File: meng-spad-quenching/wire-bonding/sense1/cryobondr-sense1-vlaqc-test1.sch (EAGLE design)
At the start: 28 parts, among them IC2 SENSE1, U2 SN74LVC1G34DCKT, X1 CONN-D3, X10 AQCR3_VDD2V5, X2 CONN-D5, X3 CONN-D4, X4 AQCR3_AV_DET, X5 AQCR3_IBIAS, X6 CONN-D6, X7 CONN-D7, X8 CONN-D8, X9 AQCR3_SPAD_CATHODE

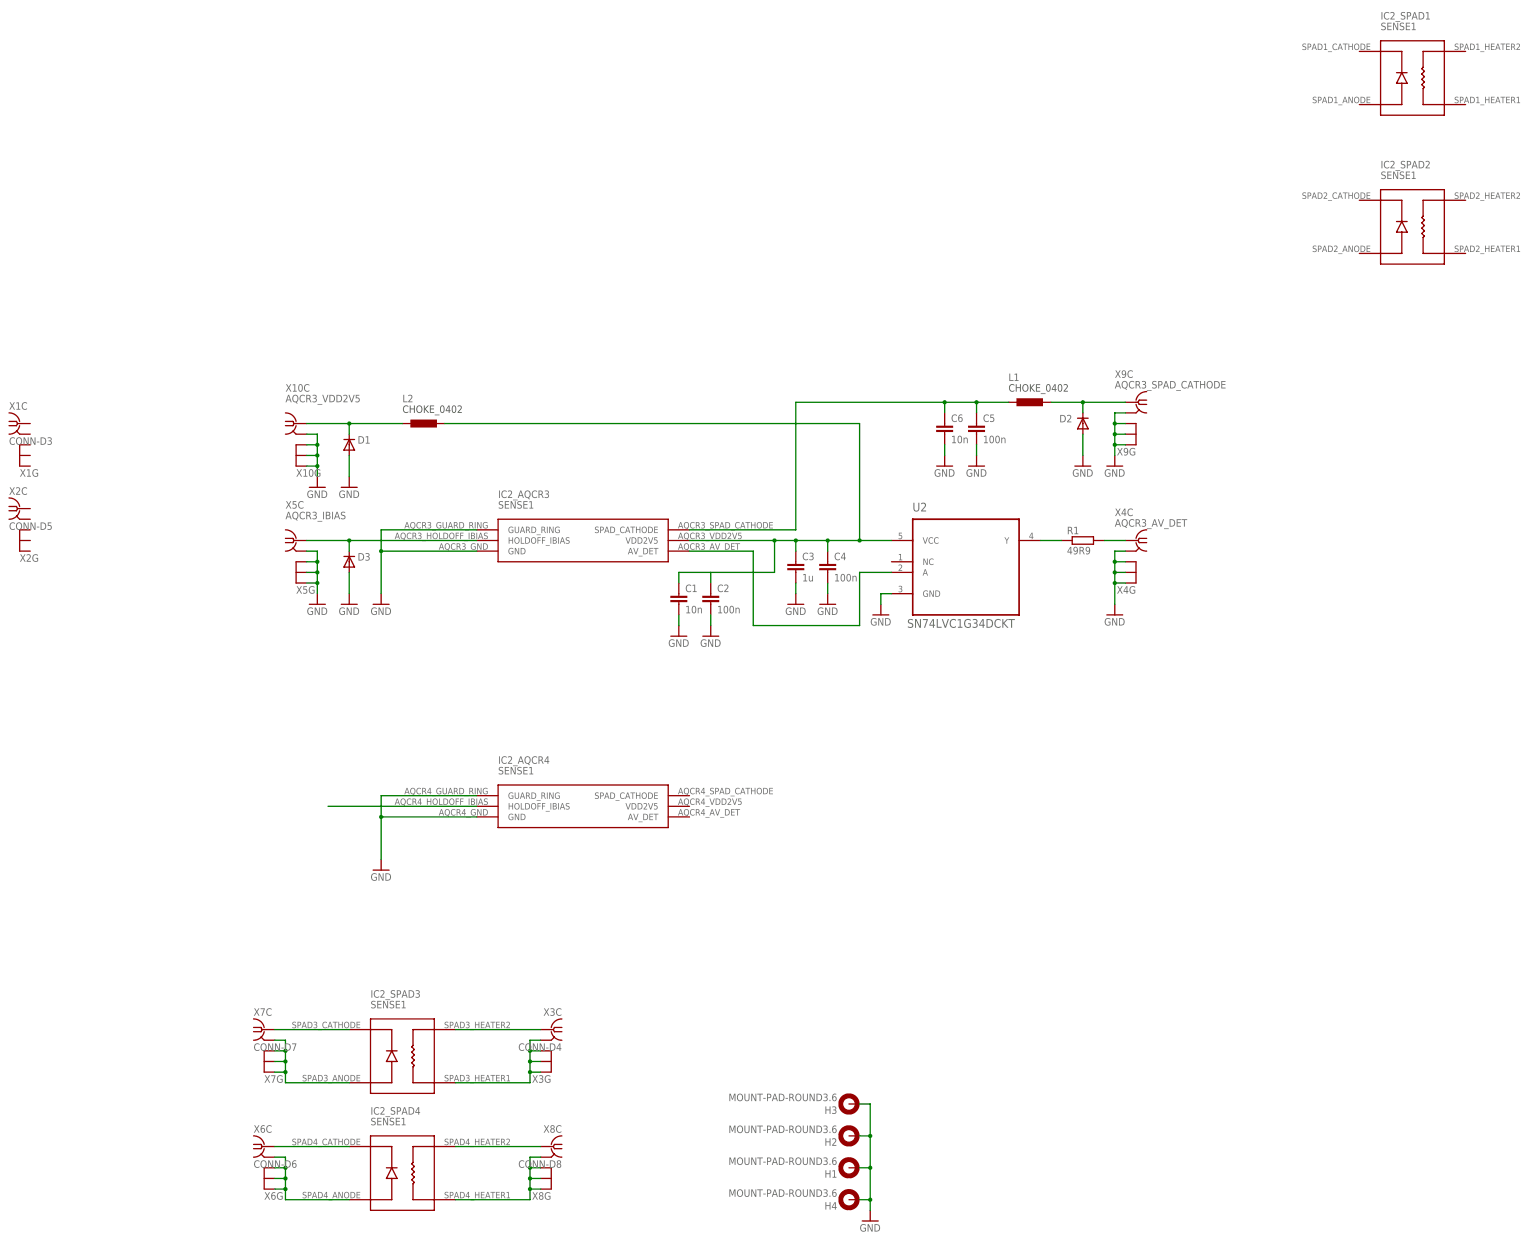
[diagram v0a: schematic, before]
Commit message: Added all MakeMIT active probe files (unsorted)
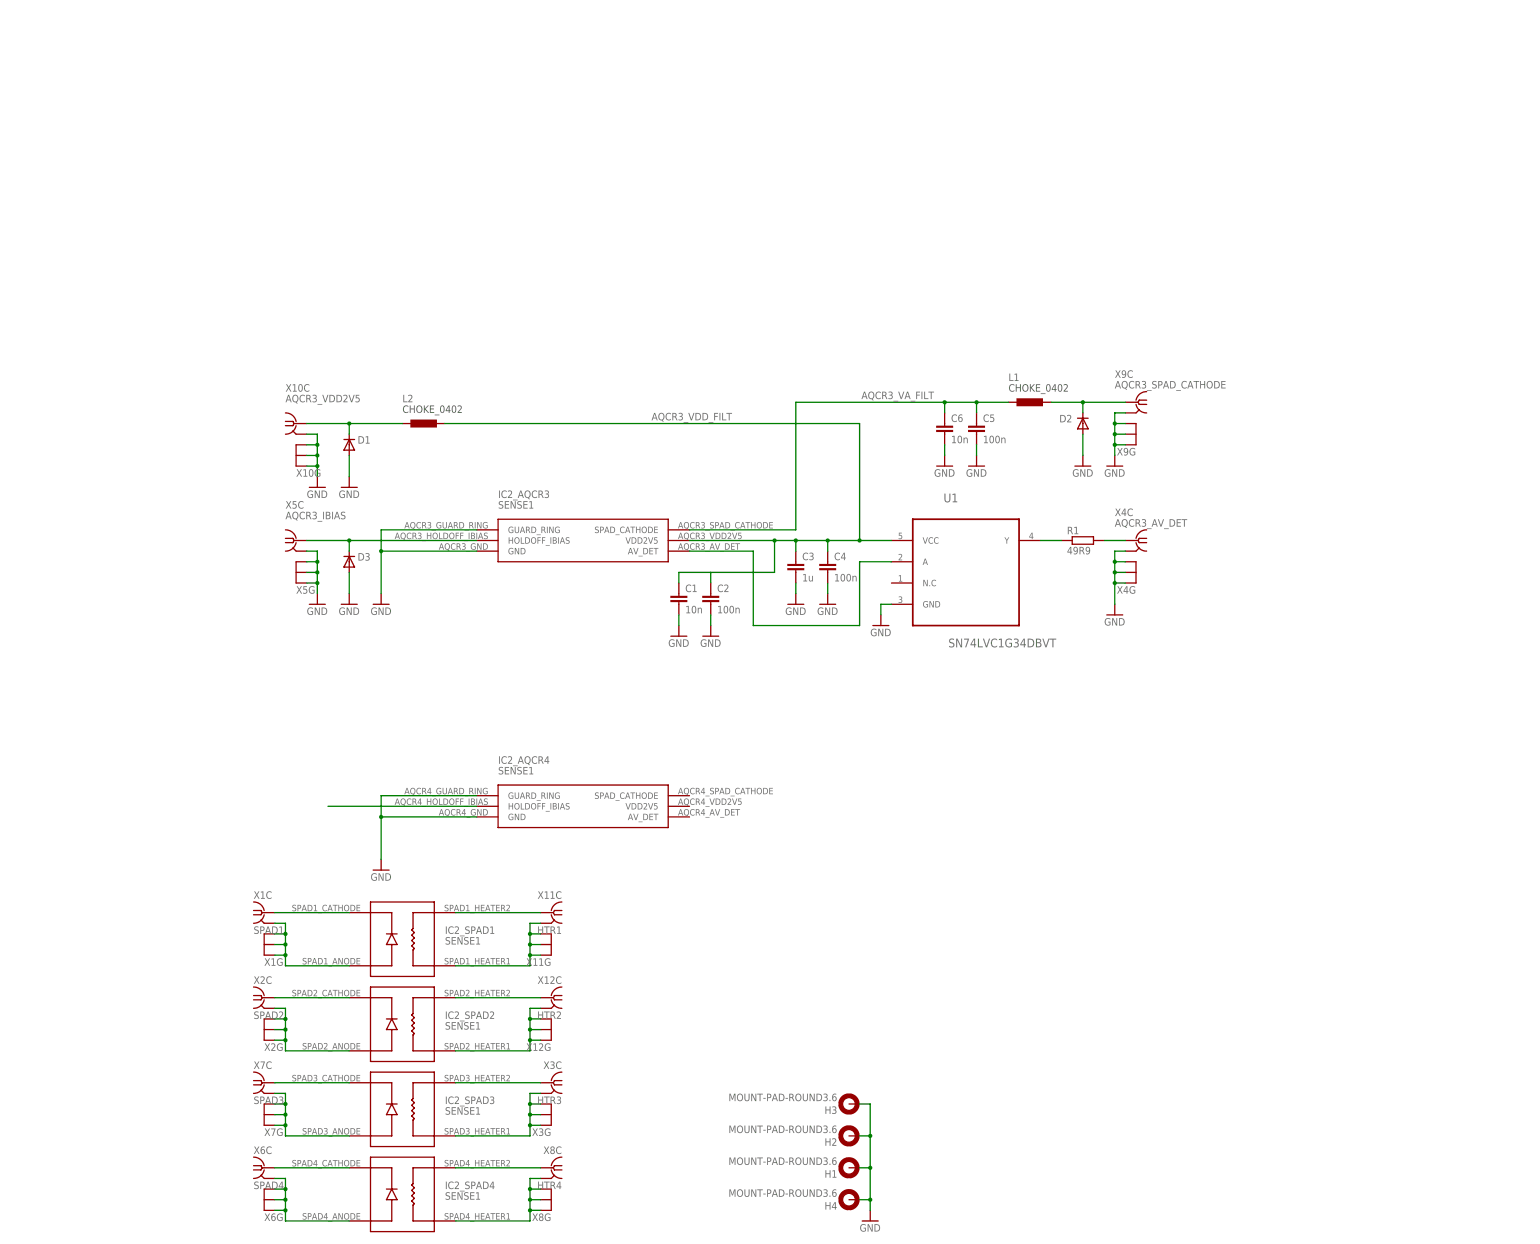
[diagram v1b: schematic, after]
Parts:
- removed U2: SN74LVC1G34DCKT, Texas Instruments_By_element14_Batch_1:SN74LVC1G34DCKT
- added U1: SN74LVC1G34DBVT, Texas Instruments_By_element14_Batch_1:SN74LVC1G34DBVT
- added X11: HTR1, meng:MMCXBIGPAD
- added X12: HTR2, meng:MMCXBIGPAD
- C1, C2, C3, C4, C5, C6: device rcl:C-EUC0402 -> rcl:C-EUC0603
- D1, D2, D3: device diode:DIODE-SOD123 -> diode:DIODE-SOD323-W
- X1: value CONN-D3 -> SPAD1
- X2: value CONN-D5 -> SPAD2
- X3: value CONN-D4 -> HTR3
- X6: value CONN-D6 -> SPAD4
- X7: value CONN-D7 -> SPAD3
- X8: value CONN-D8 -> HTR4
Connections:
- net N$8 renamed AQCR3_VA_FILT
- removed net N$9: C1.1, C2.1, C3.1, C4.1, IC2_AQCR3.VDD2V5, L2.P$2, U2.VCC
- new net AQCR3_VDD_FILT: C1.1, C2.1, C3.1, C4.1, IC2_AQCR3.VDD2V5, L2.P$2, U1.VCC
- new net N$18: IC2_SPAD2.SPAD_CATHODE, X2C.1
- new net N$19: IC2_SPAD2.SPAD_ANODE, X2C.GND, X2G.GND@1, X2G.GND@2, X2G.GND@3
- new net N$20: IC2_SPAD1.SPAD_ANODE, X1C.GND, X1G.GND@1, X1G.GND@2, X1G.GND@3
- new net N$21: IC2_SPAD1.SPAD_CATHODE, X1C.1
- new net N$22: IC2_SPAD1.SPAD_HEATER2, X11C.1
- new net N$23: IC2_SPAD2.SPAD_HEATER2, X12C.1
- new net N$24: IC2_SPAD1.SPAD_HEATER1, X11C.GND, X11G.GND@1, X11G.GND@2, X11G.GND@3
- new net N$25: IC2_SPAD2.SPAD_HEATER1, X12C.GND, X12G.GND@1, X12G.GND@2, X12G.GND@3
- net GND: now also U1.GND; no longer U2.GND
- net N$2: now also U1.Y; no longer U2.Y
- net N$7: now also U1.A; no longer U2.A
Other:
- note added: "Low-Temperature Component Guidelines: - Use NP0 tempco. ceramic capacitors or silicon capacitors (eg. IPDiA) - Use thin-film chip resistors (eg. Vishay VSMP series)"
- moved on the sheet: IC2_SPAD1, IC2_SPAD2, IC2_SPAD3, IC2_SPAD4, X1C, X1G, X2C, X2G, X3C, X3G, X6C, X6G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

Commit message: Updated R and C component packages
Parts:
- C1, C2, C3, C4, C5, C6: device rcl:C-EUC0603 -> rcl-modified-footprints:C-EUC0603
- R1: device rcl:R-EU_R0402 -> rcl-modified-footprints:R-EU_R0603
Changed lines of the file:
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@@
 <setting verticaltext="up"/>
 </settings>
-<grid distance="0.1" unitdist="inch" unit="inch" style="lines" multiple="1" display="yes" altdistance="0.01" altunitdist="inch" altunit="inch"/>
+<grid distance="0.1" unitdist="inch" unit="inch" style="lines" multiple="1" display="no" altdistance="0.01" altunitdist="inch" altunit="inch"/>
 <layers>
 <layer number="1" name="Top" color="4" fill="1" visible="yes" active="no"/>
@@
 <part name="GND1" library="supply1" deviceset="GND" device=""/>
 <part name="GND2" library="supply1" deviceset="GND" device=""/>
-<part name="C1" library="rcl" library_urn="urn:adsk.eagle:library:334" deviceset="C-EU" device="C0603" package3d_urn="urn:adsk.eagle:package:23616/2" value="10n"/>
-<part name="C2" library="rcl" library_urn="urn:adsk.eagle:library:334" deviceset="C-EU" device="C0603" package3d_urn="urn:adsk.eagle:package:23616/2" value="100n"/>
+<part name="C1" library="rcl-modified-footprints" deviceset="C-EU" device="C0603" package3d_urn="urn:adsk.eagle:package:23616/2" value="10n"/>
+<part name="C2" library="rcl-modified-footprints" deviceset="C-EU" device="C0603" package3d_urn="urn:adsk.eagle:package:23616/2" value="100n"/>
 <part name="GND3" library="supply1" deviceset="GND" device=""/>
 <part name="GND4" library="supply1" deviceset="GND" device=""/>
@@
 <attribute name="SPICEPREFIX" value="G"/>
 </part>
-<part name="C3" library="rcl" library_urn="urn:adsk.eagle:library:334" deviceset="C-EU" device="C0603" package3d_urn="urn:adsk.eagle:package:23616/2" value="1u"/>
-<part name="C4" library="rcl" library_urn="urn:adsk.eagle:library:334" deviceset="C-EU" device="C0603" package3d_urn="urn:adsk.eagle:package:23616/2" value="100n"/>
+<part name="C3" library="rcl-modified-footprints" deviceset="C-EU" device="C0603" package3d_urn="urn:adsk.eagle:package:23616/2" value="1u"/>
+<part name="C4" library="rcl-modified-footprints" deviceset="C-EU" device="C0603" package3d_urn="urn:adsk.eagle:package:23616/2" value="100n"/>
 <part name="GND6" library="supply1" deviceset="GND" device=""/>
 <part name="GND7" library="supply1" deviceset="GND" device=""/>
 <part name="GND8" library="supply1" deviceset="GND" device=""/>
 <part name="GND9" library="supply1" deviceset="GND" device=""/>
-<part name="R1" library="rcl" library_urn="urn:adsk.eagle:library:334" deviceset="R-EU_" device="R0402" package3d_urn="urn:adsk.eagle:package:23547/1" value="49R9"/>
+<part name="R1" library="rcl-modified-footprints" deviceset="R-EU_" device="R0603" package3d_urn="urn:adsk.eagle:package:23555/2" value="49R9"/>
 <part name="X9" library="meng" deviceset="MMCX" device="BIGPAD" value="AQCR3_SPAD_CATHODE"/>
 <part name="GND10" library="supply1" deviceset="GND" device=""/>
@@
 <part name="GND12" library="supply1" deviceset="GND" device=""/>
 <part name="GND13" library="supply1" deviceset="GND" device=""/>
-<part name="C5" library="rcl" library_urn="urn:adsk.eagle:library:334" deviceset="C-EU" device="C0603" package3d_urn="urn:adsk.eagle:package:23616/2" value="100n"/>
-<part name="C6" library="rcl" library_urn="urn:adsk.eagle:library:334" deviceset="C-EU" device="C0603" package3d_urn="urn:adsk.eagle:package:23616/2" value="10n"/>
+<part name="C5" library="rcl-modified-footprints" deviceset="C-EU" device="C0603" package3d_urn="urn:adsk.eagle:package:23616/2" value="100n"/>
+<part name="C6" library="rcl-modified-footprints" deviceset="C-EU" device="C0603" package3d_urn="urn:adsk.eagle:package:23616/2" value="10n"/>
 <part name="GND14" library="supply1" deviceset="GND" device=""/>
 <part name="GND15" library="supply1" deviceset="GND" device=""/>
